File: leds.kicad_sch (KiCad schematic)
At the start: 22 parts, among them U2 AMS1117-5.0

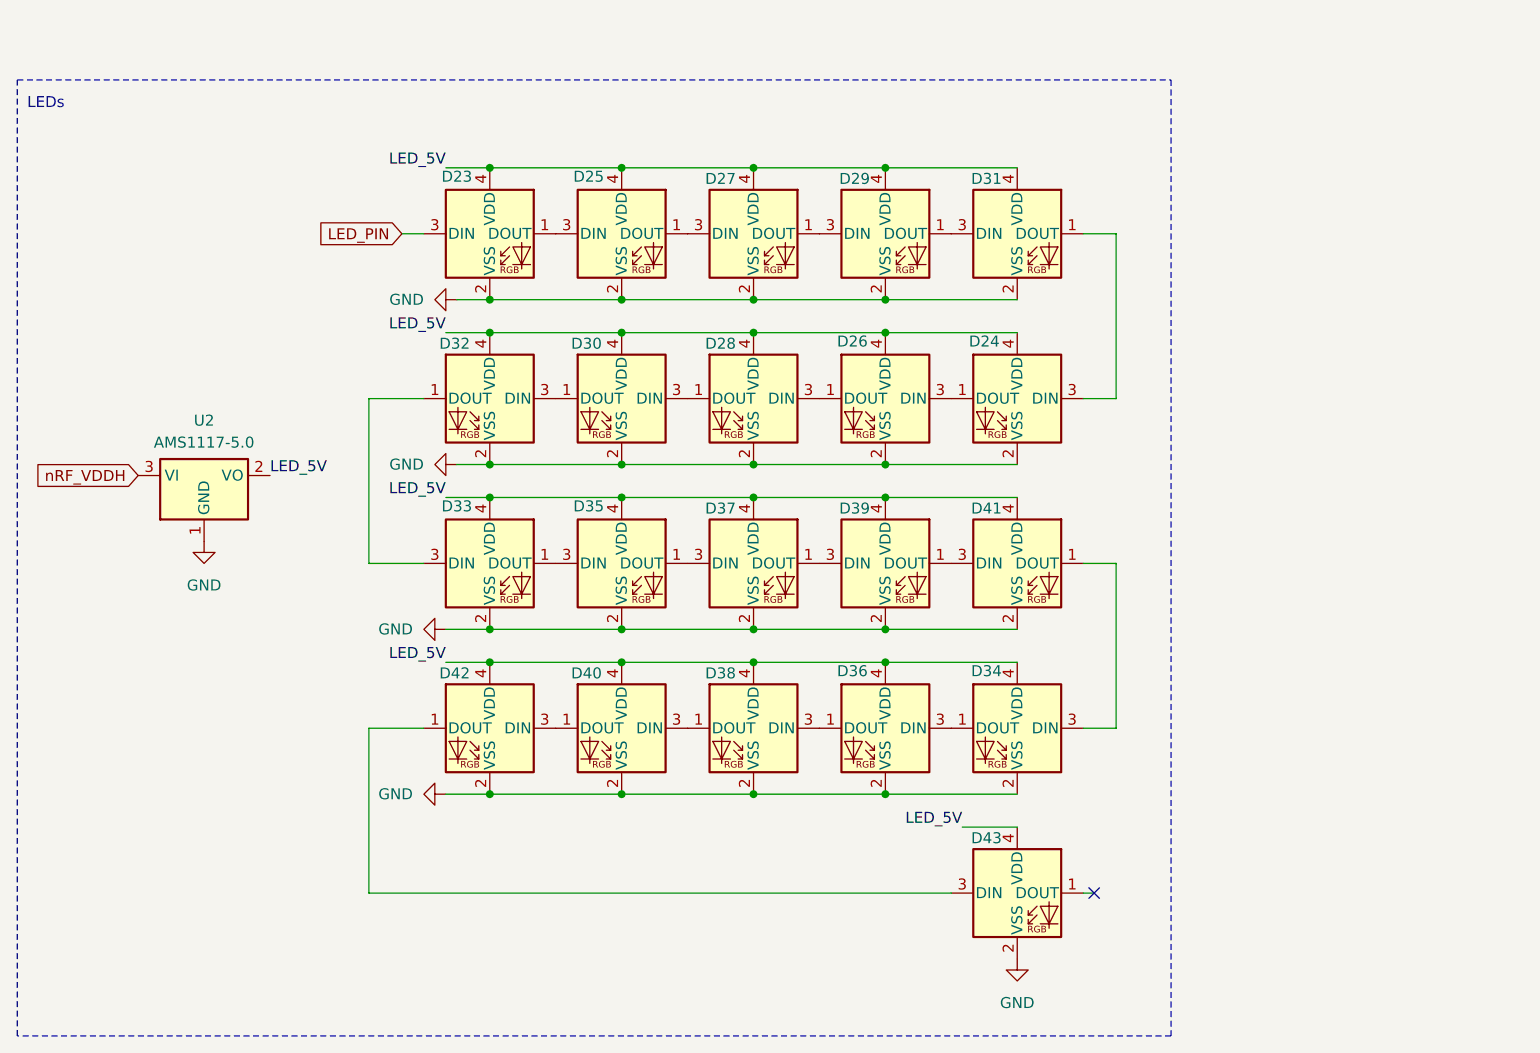
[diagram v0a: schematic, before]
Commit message: before auto route
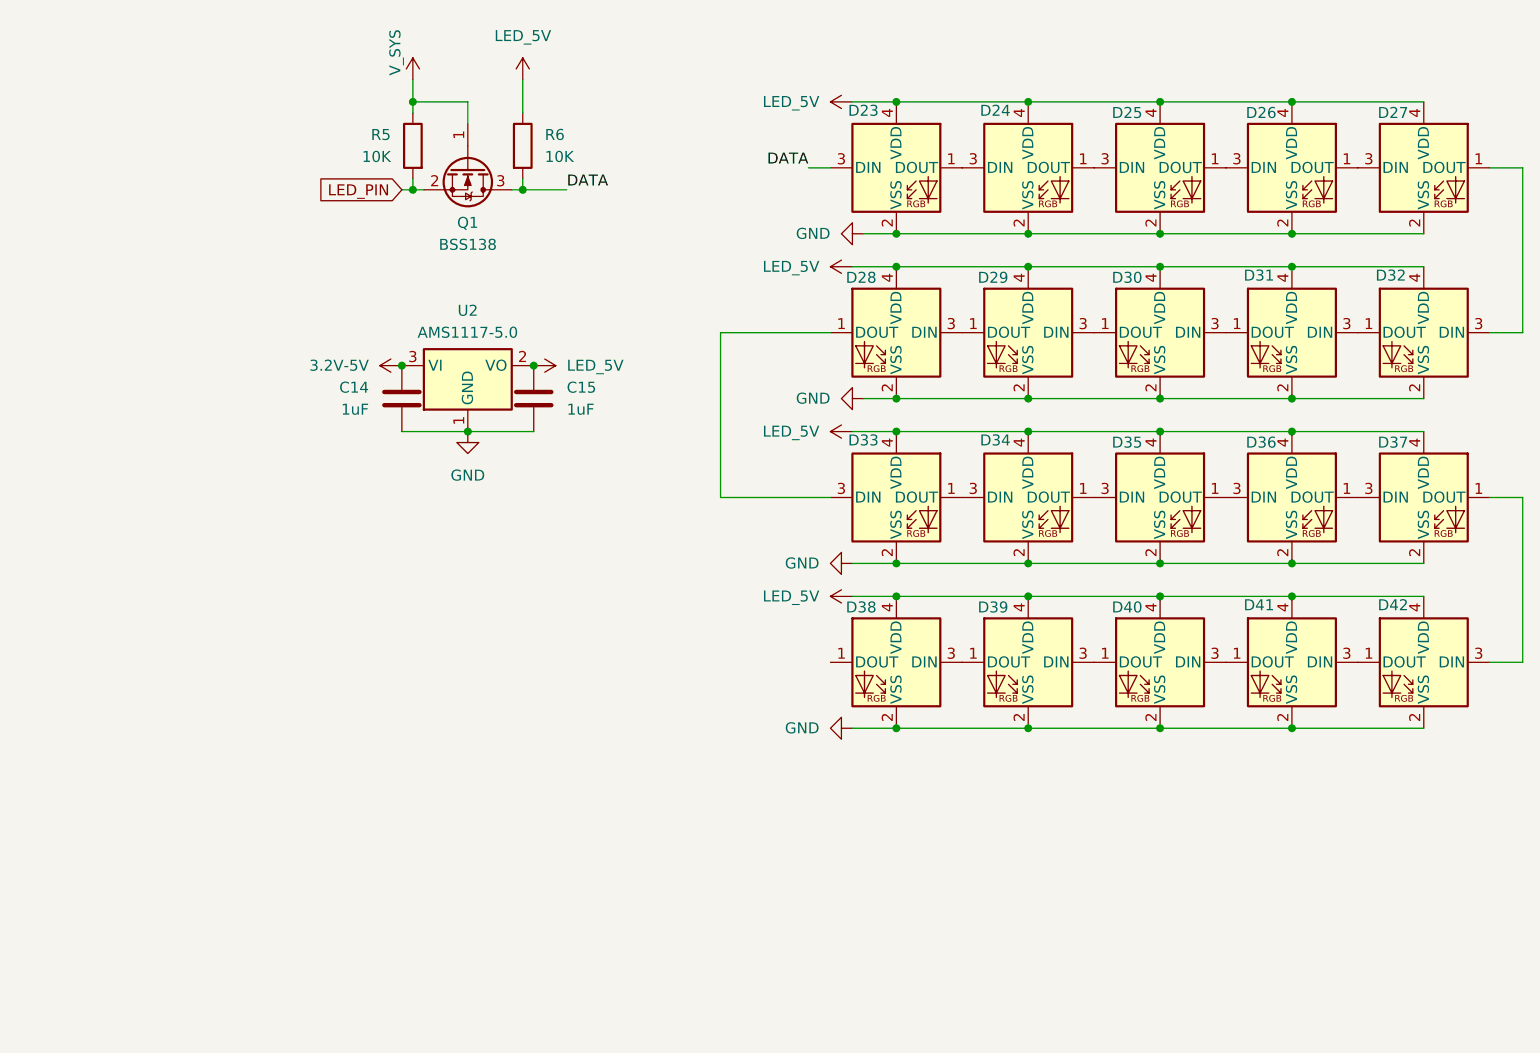
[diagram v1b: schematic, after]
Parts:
- removed D43: WS2812B-2020, LED_SMD:LED_WS2812B_PLCC4_5.0x5.0mm_P3.2mm, symbol LED:WS2812B-2020
- added C14, C15: 1uF, Capacitor_SMD:C_0402_1005Metric, symbol Device:C
- added Q1: BSS138, Package_TO_SOT_SMD:SOT-23, symbol Transistor_FET:BSS138
- added R5, R6: 10K, Resistor_SMD:R_0201_0603Metric, symbol Device:R
- renumbered D25 to D24, D27 to D25, D29 to D26, D31 to D27, D32 to D28, D30 to D29, D28 to D30, D26 to D31, D24 to D32, D35 to D34, D37 to D35, D39 to D36, D41 to D37, D42 to D38, D40 to D39, D38 to D40, D36 to D41, D34 to D42
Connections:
- net GND: now also C14.2, C15.2
- net LED_5V: now also C15.1, R6.1
- net LED_PIN: now also Q1.2 (S), R5.2; no longer D23.3 (DIN)
- net nRF_VDDH renamed 3.2V-5V
- net 3.2V-5V: now also C14.1
- new net DATA: D23.3 (DIN), Q1.3 (D), R6.2
- new net V_SYS: Q1.1 (G), R5.1
- no-connect marks 1 -> 0
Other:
- note removed: "LEDs"
- moved on the sheet: D23, D24, D25, D26, D27, D28, D29, D30, D31, D32, D33, D34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
